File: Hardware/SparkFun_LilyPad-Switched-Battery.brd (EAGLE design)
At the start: 29.4 x 29.2 mm, 12 parts

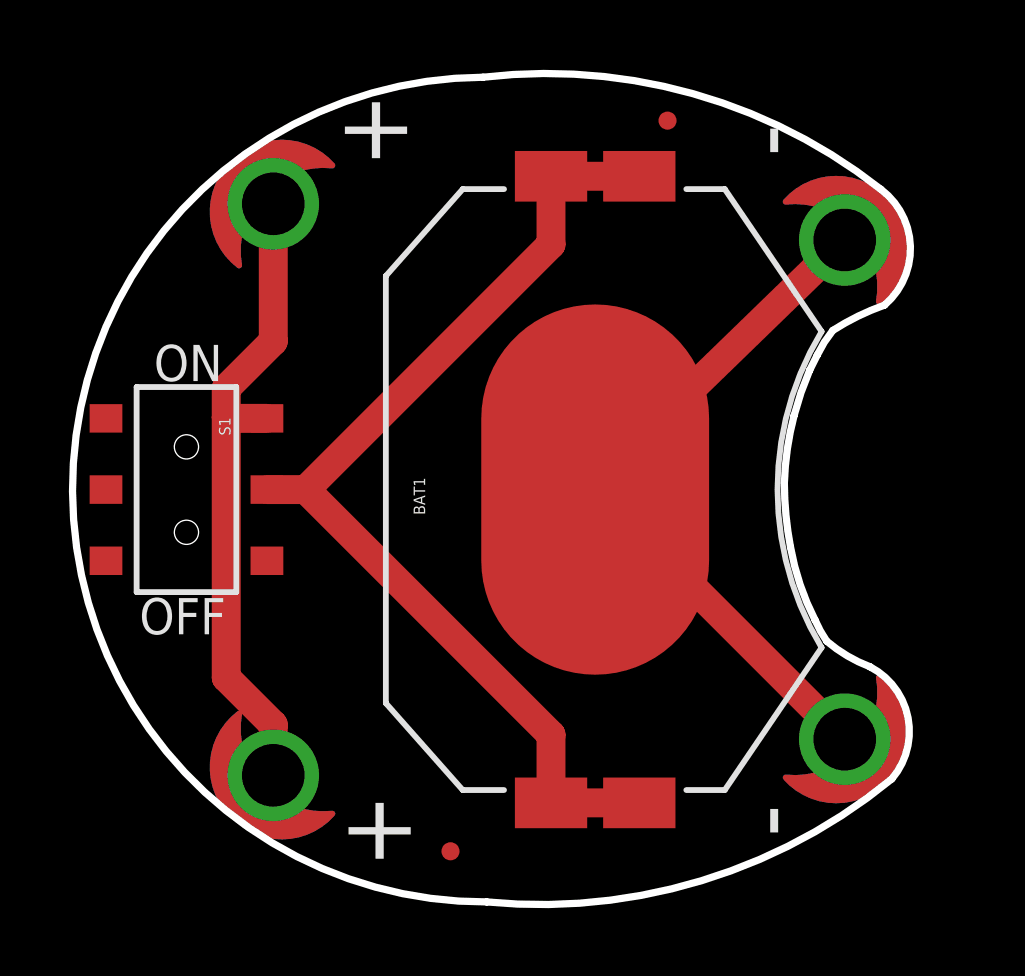
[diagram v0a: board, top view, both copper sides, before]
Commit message: resolving merge conflicts - again
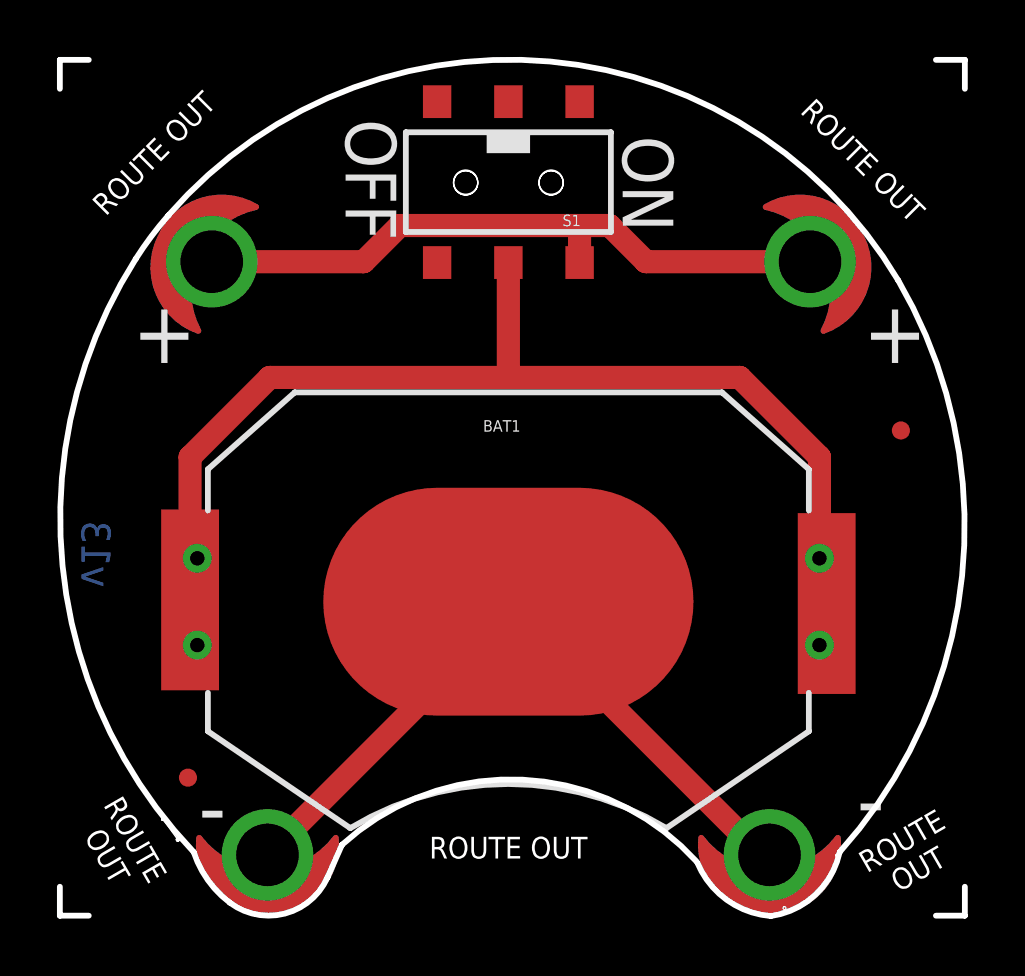
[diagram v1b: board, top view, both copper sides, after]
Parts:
- removed JP1, JP2: FIDUCIALUFIDUCIAL, SparkFun:MICRO-FIDUCIAL
- removed U$2, U$4: SEWTAP6, LilyPad-Wearables:PETAL-SMALL-2SIDE
- removed U$5: LOGO-LPLP, LilyPad-Wearables:LOGO-LILYPAD
- removed U$7: OSHW-LOGOS, SparkFun-Aesthetics:OSHW-LOGO-S
- removed U$8: CREATIVE_COMMONS, SparkFun-Aesthetics:CREATIVE_COMMONS
- added BATB-, BATB-2, BATT+, BATT+2: SEWTAP6, LilyPad-Wearables:PETAL-SMALL-2SIDE
- added FD1, FD2: FIDUCIALUFIDUCIAL, SparkFun-Aesthetics:MICRO-FIDUCIAL
- added FRAME1: FRAME-LETTER, SparkFun-Aesthetics:CREATIVE_COMMONS
- added LOGO2: OSHW-LOGOS, SparkFun-Aesthetics:OSHW-LOGO-S
- BAT1: value (none) -> 20mm coincell
- LOGO1: value SPECIAL_INSTRUCTIONS-ORDERING -> SFE_LOGO_FLAME.1_INCH; device SparkFun-Aesthetics:ORDERING_INSTRUCTIONS -> SparkFun-Aesthetics:SFE_LOGO_FLAME_.1
- S1: device SparkFun:AYZ0202 -> SparkFun-Electromechanical:AYZ0202
- U$1: value SEWTAP6 -> REVISION; device LilyPad-Wearables:PETAL-SMALL-2SIDE -> SparkFun-Aesthetics:REVISION
- U$3: value SEWTAP6 -> (none); device LilyPad-Wearables:PETAL-SMALL-2SIDE -> LilyPad-Wearables:LOGO-LILYPAD
- moved LOGO1 43.7 mm to (11.6, 24.8), flipped to the bottom
- moved U$1 31.4 mm to (2.42, -12.0), turned to 0 degrees
- moved S1 15.6 mm to (16.0, 26.0), turned to 180 degrees
- moved U$3 15.1 mm to (15.8, 14.9), flipped to the bottom, turned to 0 degrees
- moved BAT1 4.98 mm to (16.0, 11.3), turned to 0 degrees
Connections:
- removed net N$3: BAT1.1, BAT1.3, BAT1.P$1, BAT1.P$2, S1.2
- new net GND: BAT1.NEGATIVE, BATB-.1, BATB-2.1
- net N$1: now also BAT1.POSITIVE@1, BAT1.POSITIVE@2, BAT1.POSITIVE@3, BAT1.POSITIVE@4, S1.2; no longer S1.1, U$2.1, U$4.1
- net N$2: now also BATT+.1, BATT+2.1, S1.1; no longer BAT1.2, U$1.1, U$3.1
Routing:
- net N$3: track 36.7 -> 0.00 mm
- net GND: track 0.00 -> 25.2 mm
- net N$1: track 22.9 -> 46.5 mm, vias 0 -> 4
- net N$2: track 26.1 -> 23.4 mm
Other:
- board size 29.4 x 29.2 mm -> 31.8 x 30.1 mm
- board text added: "All Units Inches"
- board text added: "Board Thickness: 0.8mm"
- board text added: "Jim Lindblom"
- board text added: "M. West"
- board text added: "Purple Solder Mask"
- board text added: "ROUTE OUT"
- board text added: "Switched Coin Cell Battery Holder"
- board text added: "v13"
- board text removed: "Board Thickness is 0.8mm"
